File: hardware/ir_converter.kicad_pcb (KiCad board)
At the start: 2 copper layers, 38.1 x 53.1 mm, 46 parts, among them J1 MX-47346-0001, J2 SWD, J3 TP, J4 TP, Q1 LL-S350PTC-1A, Q2 BC817-40, SW1 RESET, SW2 SW2, U1 TLV70033DDCT, U2 USBLC6-2, U3 STM32F103C8T6

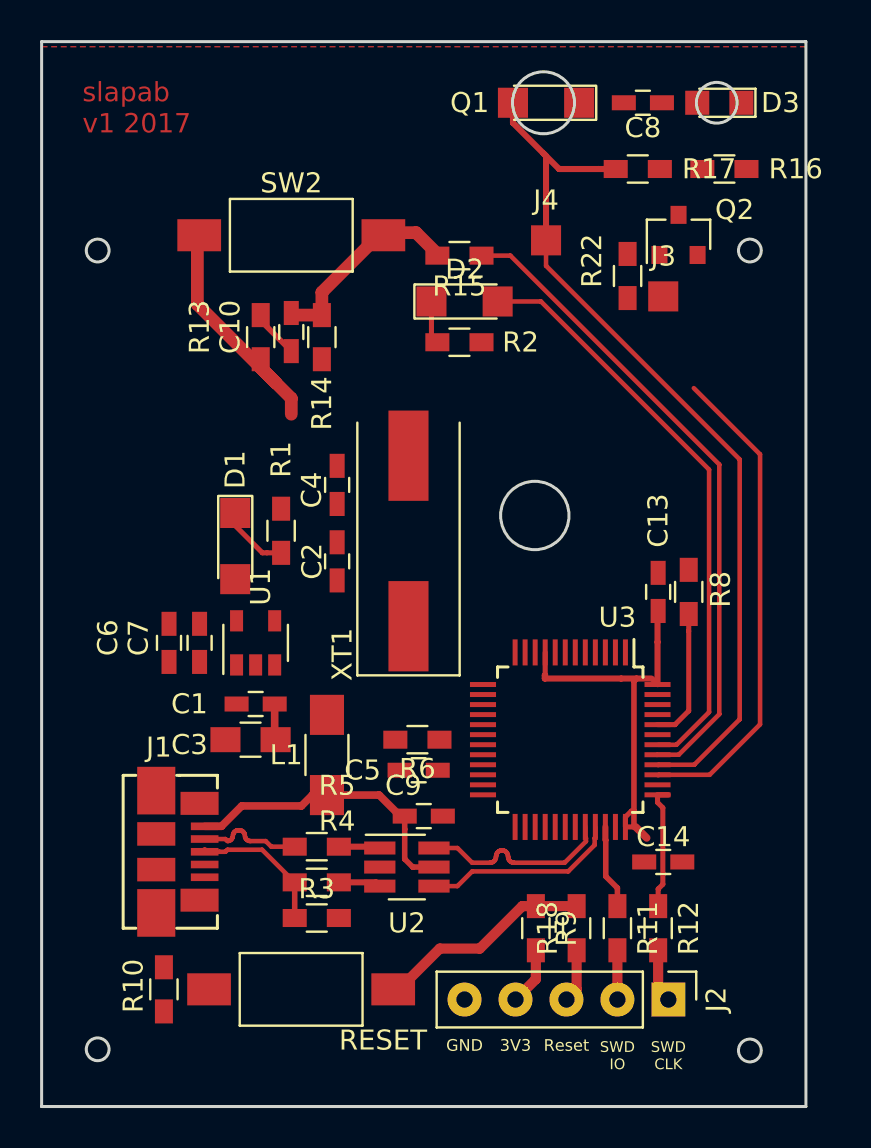
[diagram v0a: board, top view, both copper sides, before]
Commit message: Almost done.
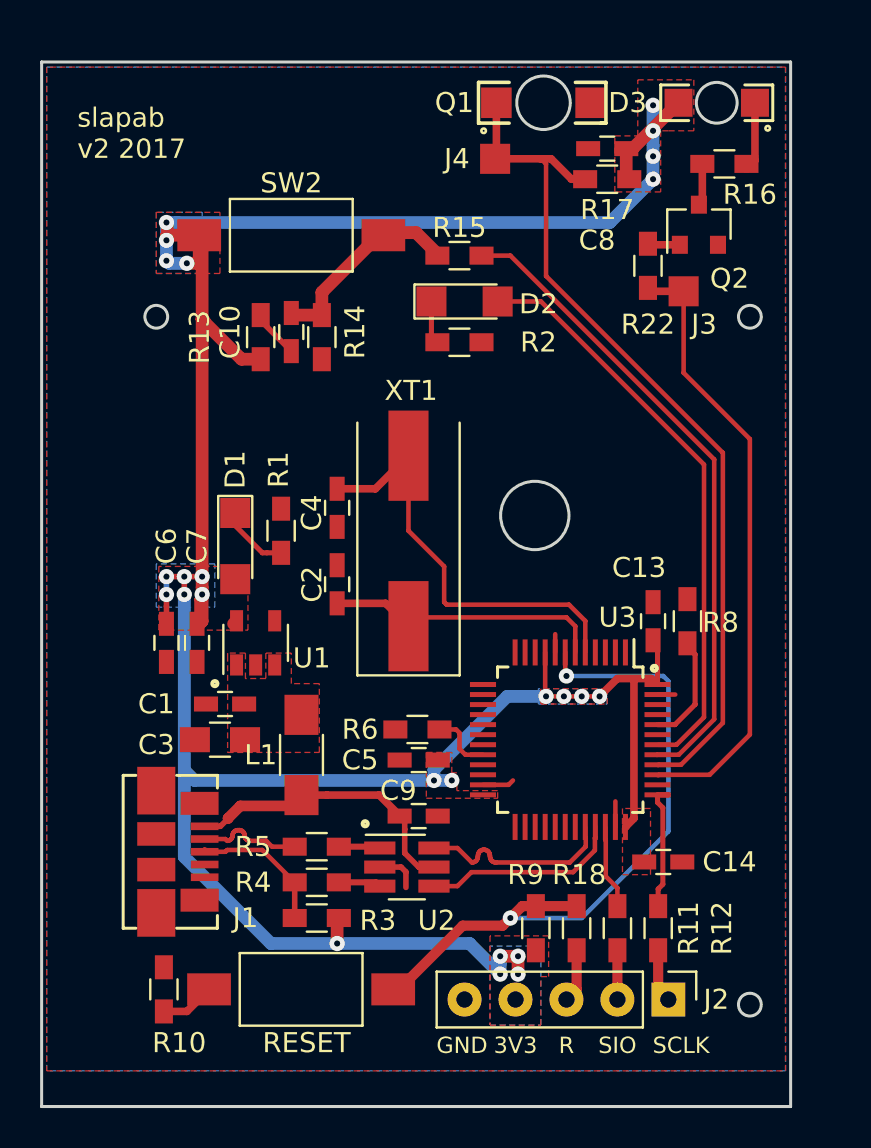
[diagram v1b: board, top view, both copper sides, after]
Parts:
- D3: footprint LEDs:LED_0805 -> CustomFootprints:IR_LED_WIDE
- Q1: footprint LEDs:LED_1206 -> CustomFootprints:IR_PHOTO_WIDE
- moved J4 4.79 mm to (100.1, 94.5)
- moved C8 2.90 mm to (105.7, 94.0)
- moved R17 1.61 mm to (105.7, 95.5)
- moved C1 1.52 mm to (86.6, 121.7)
- moved C3 1.52 mm to (86.4, 123.4)
- moved C13 1.48 mm to (108.0, 117.5)
- moved R8 1.46 mm to (109.7, 117.5)
- moved L1 1.27 mm to (90.4, 124.2)
- moved C2 1.14 mm to (92.2, 115.7)
- moved C4 1.14 mm to (92.2, 111.9)
- moved Q2 1.14 mm to (110.2, 97.8)
- moved R22 1.14 mm to (107.7, 99.8)
- moved J3 1.05 mm to (109.5, 101.1)
- moved C5 0.51 mm to (96.3, 124.5)
- moved R6 0.51 mm to (96.2, 122.9)
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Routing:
- net +3V3: track 35.4 -> 147.2 mm, vias 0 -> 25
- net /RESET: track 10.9 -> 34.4 mm, vias 0 -> 2
- net /OSC_IN: track 0.00 -> 21.3 mm
- net /OSC_OUT: track 0.00 -> 14.0 mm
- net GND: track 0.00 -> 6.83 mm
- net /IR_CLK: track 24.3 -> 30.7 mm
- net Net-(D3-Pad1): track 0.00 -> 3.48 mm
- net /BOOT1: track 0.00 -> 3.16 mm
- net Net-(R10-Pad1): track 0.00 -> 2.71 mm
- net Net-(Q2-Pad3): track 0.00 -> 1.85 mm
- net Net-(Q2-Pad1): track 0.00 -> 1.61 mm
- net /BOOT0: track 6.67 -> 5.60 mm
- net +5V: track 1.80 -> 0.83 mm
- net /IR_IN: track 44.3 -> 43.7 mm
- added copper zone on B.Cu, net +3V3
- added copper zone on F.Cu, net +3V3
- added copper zone on F.Cu, net +5V
- added copper zone on B.Cu, net GND
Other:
- board size 38.1 x 53.1 mm -> 37.3 x 52.1 mm
- net class 3v3: via_dia 0.889 -> 0.762
- net class Default: via_dia 0.889 -> 0.762
- rule via_min_size: 0.5 -> 0.635
- board text added: "R"
- board text added: "SCLK"
- board text added: "SIO"
- board text added: "slapab v2 2017"
- board text removed: "Reset"
- board text removed: "SWD CLK"
- board text removed: "SWD IO"
- board text removed: "slapab v1 2017"
